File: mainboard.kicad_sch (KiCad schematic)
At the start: 15 parts, among them IC1 AZ1117CH-3.3TRG1, P1 OKLT6W12NC, U1 MCP2517FD-xSL, U5 MCP2517FD-xSL

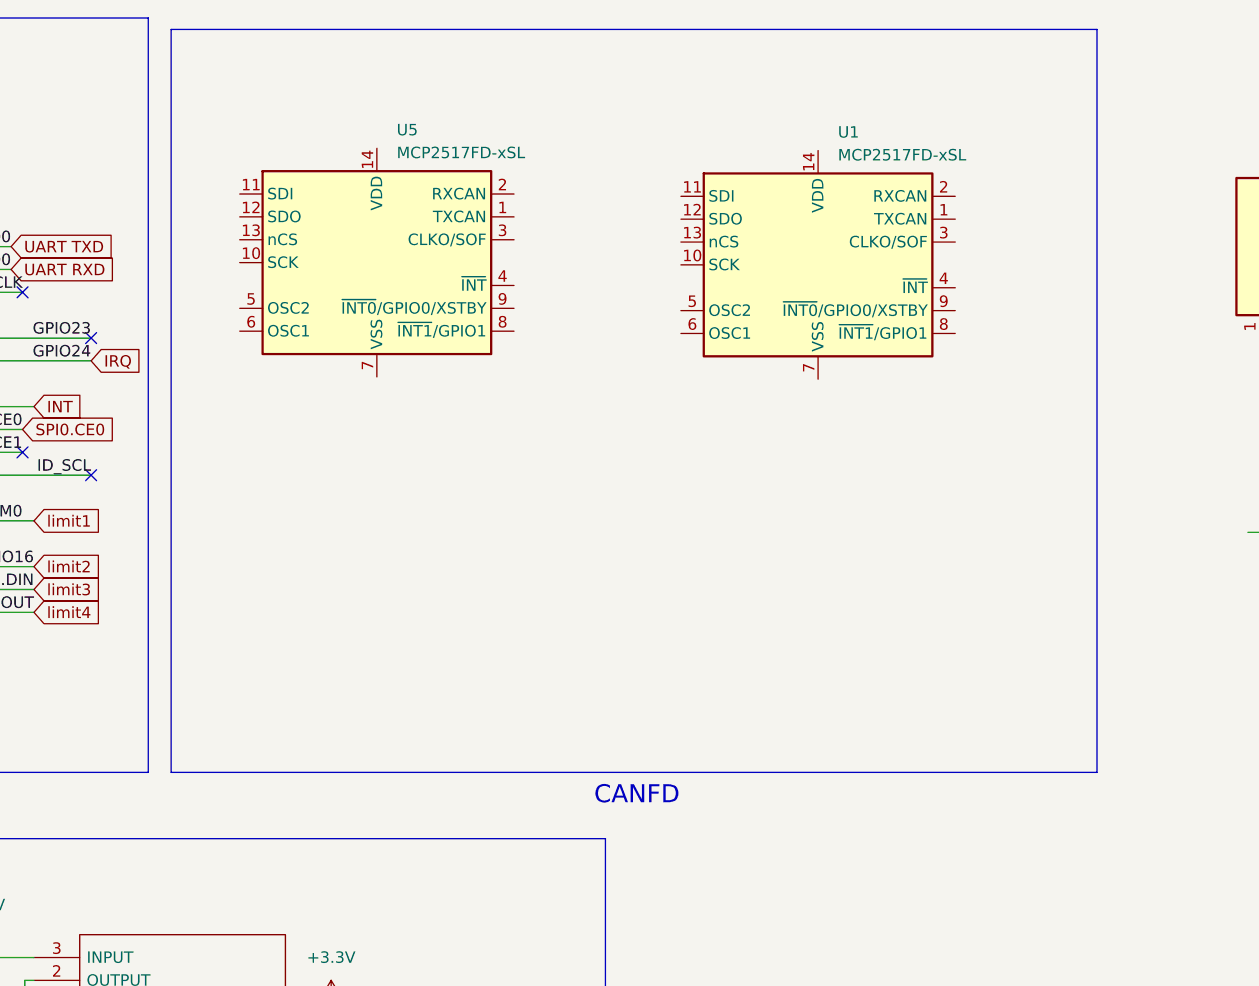
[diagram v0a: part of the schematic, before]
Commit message: 更新
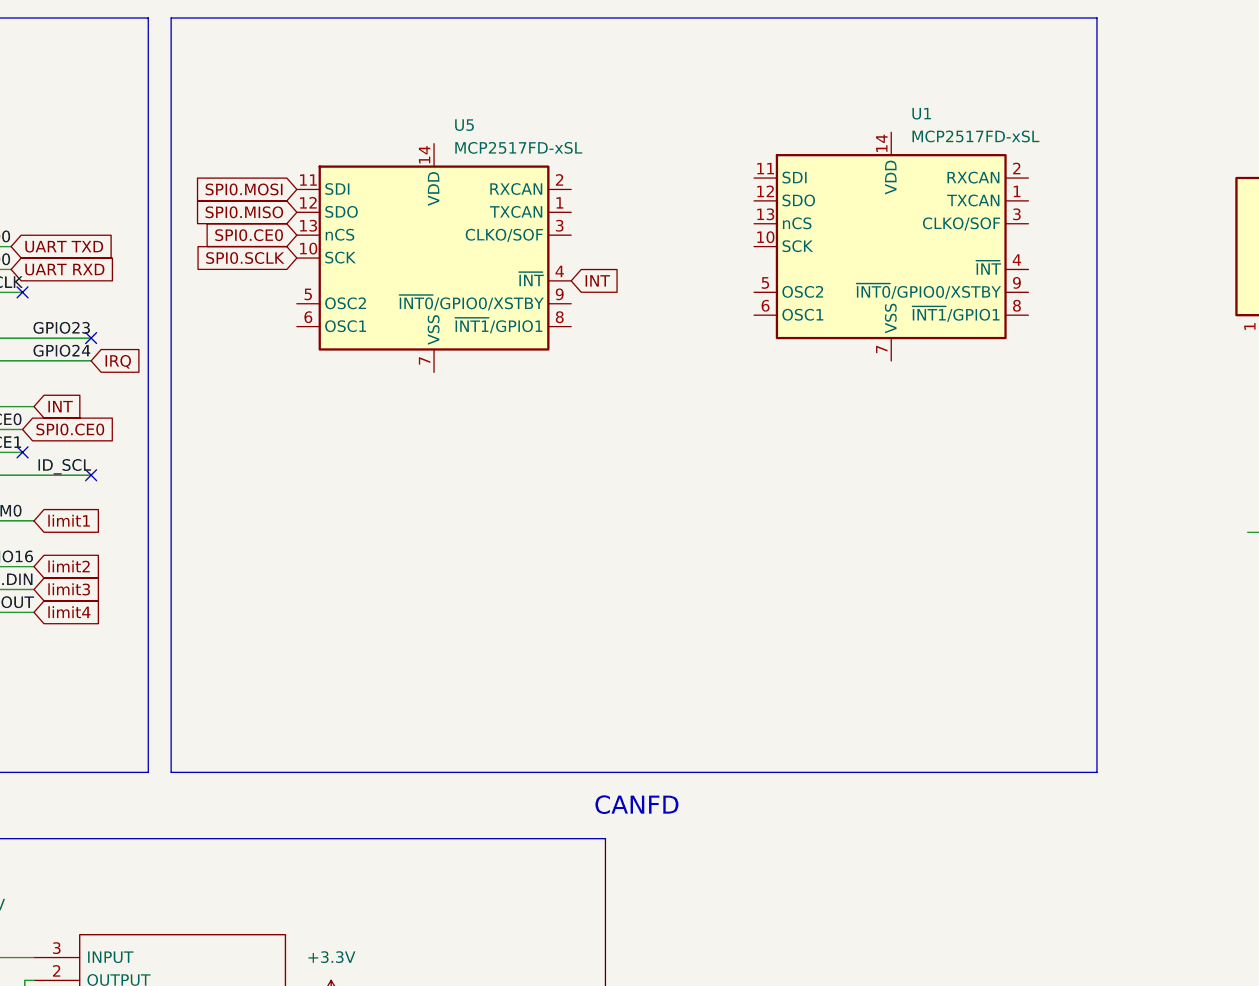
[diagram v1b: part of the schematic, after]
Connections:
- net INT: now also U5.4 (~{INT})
- net SPI0.CE0: now also U5.13 (nCS)
- net SPI0.MISO: now also U5.12 (SDO)
- net SPI0.MOSI: now also U5.11 (SDI)
- net SPI0.SCLK: now also U5.10 (SCK)
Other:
- moved on the sheet: U1, U5
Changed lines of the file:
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@@
     (fill (type none))
   )
-  (rectangle (start 100.33 19.05) (end 203.2 101.6)
+  (rectangle (start 100.33 17.78) (end 203.2 101.6)
     (stroke (width 0) (type default))
     (fill (type none))
@@
     (effects (font (size 2 2)) (justify left bottom))
   )
-  (text "CANFD" (at 147.32 105.41 0)
+  (text "CANFD" (at 147.32 106.68 0)
     (effects (font (size 2 2)) (justify left bottom))
   )
@@
     )
   )
+  (global_label "SPI0.SCLK" (shape input) (at 114.3 44.45 180) (fields_autoplaced)
+    (effects (font (size 1.27 1.27)) (justify right))
+    (property "Intersheetrefs" "${INTERSHEET_REFS}" (at 101.6386 44.45 0)
+      (effects (font (size 1.27 1.27)) (justify right) hide)
+    )
+  )
+  (global_label "INT" (shape input) (at 144.78 46.99 0) (fields_autoplaced)
+    (effects (font (size 1.27 1.27)) (justify left))
+    (property "Intersheetrefs" "${INTERSHEET_REFS}" (at 150.6681 46.99 0)
+      (effects (font (size 1.27 1.27)) (justify left) hide)
+    )
+  )
   (global_label "LED_R" (shape input) (at 22.86 50.8 180) (fields_autoplaced)
     (effects (font (size 1.27 1.27)) (justify right))
@@
     )
   )
+  (global_label "SPI0.CE0" (shape input) (at 114.3 41.91 180) (fields_autoplaced)
+    (effects (font (size 1.27 1.27)) (justify right))
+    (property "Intersheetrefs" "${INTERSHEET_REFS}" (at 102.7877 41.91 0)
+      (effects (font (size 1.27 1.27)) (justify right) hide)
+    )
+  )
+  (global_label "SPI0.MISO" (shape input) (at 114.3 39.37 180) (fields_autoplaced)
+    (effects (font (size 1.27 1.27)) (justify right))
+    (property "Intersheetrefs" "${INTERSHEET_REFS}" (at 101.82 39.37 0)
+      (effects (font (size 1.27 1.27)) (justify right) hide)
+    )
+  )
   (global_label "SPI0.CE0" (shape input) (at 83.82 63.5 0) (fields_autoplaced)
     (effects (font (size 1.27 1.27)) (justify left))
@@
     (property "Intersheetrefs" "${INTERSHEET_REFS}" (at 90.9781 60.96 0)
       (effects (font (size 1.27 1.27)) (justify left) hide)
+    )
+  )
+  (global_label "SPI0.MOSI" (shape input) (at 114.3 36.83 180) (fields_autoplaced)
+    (effects (font (size 1.27 1.27)) (justify right))
+    (property "Intersheetrefs" "${INTERSHEET_REFS}" (at 101.82 36.83 0)
+      (effects (font (size 1.27 1.27)) (justify right) hide)
     )
   )
@@
     )
   )
-  (symbol (lib_id "Interface_CAN_LIN:MCP2517FD-xSL") (at 172.212 45.212 0) (unit 1)
-    (in_bom yes) (on_board yes) (dnp no) (fields_autoplaced)
-    (property "Reference" "U1" (at 174.4061 30.48 0)
-      (effects (font (size 1.27 1.27)) (justify left))
-    )
-    (property "Value" "MCP2517FD-xSL" (at 174.4061 33.02 0)
-      (effects (font (size 1.27 1.27)) (justify left))
-    )
-    (property "Footprint" "Package_SO:SOIC-14_3.9x8.7mm_P1.27mm" (at 172.212 70.612 0)
-      (effects (font (size 1.27 1.27)) hide)
-    )
-    (property "Datasheet" "https://ww1.microchip.com/downloads/en/DeviceDoc/20005688A.pdf" (at 172.212 38.862 0)
+  (symbol (lib_id "Interface_CAN_LIN:MCP2517FD-xSL") (at 180.34 43.18 0) (unit 1)
+    (in_bom yes) (on_board yes) (dnp no) (fields_autoplaced)
+    (property "Reference" "U1" (at 182.5341 28.448 0)
+      (effects (font (size 1.27 1.27)) (justify left))
+    )
+    (property "Value" "MCP2517FD-xSL" (at 182.5341 30.988 0)
+      (effects (font (size 1.27 1.27)) (justify left))
+    )
+    (property "Footprint" "Package_SO:SOIC-14_3.9x8.7mm_P1.27mm" (at 180.34 68.58 0)
+      (effects (font (size 1.27 1.27)) hide)
+    )
+    (property "Datasheet" "https://ww1.microchip.com/downloads/en/DeviceDoc/20005688A.pdf" (at 180.34 36.83 0)
       (effects (font (size 1.27 1.27)) hide)
     )
@@
     )
   )
-  (symbol (lib_id "Interface_CAN_LIN:MCP2517FD-xSL") (at 123.19 44.958 0) (unit 1)
-    (in_bom yes) (on_board yes) (dnp no) (fields_autoplaced)
-    (property "Reference" "U5" (at 125.3841 30.226 0)
-      (effects (font (size 1.27 1.27)) (justify left))
-    )
-    (property "Value" "MCP2517FD-xSL" (at 125.3841 32.766 0)
-      (effects (font (size 1.27 1.27)) (justify left))
-    )
-    (property "Footprint" "Package_SO:SOIC-14_3.9x8.7mm_P1.27mm" (at 123.19 70.358 0)
-      (effects (font (size 1.27 1.27)) hide)
-    )
-    (property "Datasheet" "https://ww1.microchip.com/downloads/en/DeviceDoc/20005688A.pdf" (at 123.19 38.608 0)
-      (effects (font (size 1.27 1.27)) hide)
-    )
+  (symbol (lib_id "Interface_CAN_LIN:MCP2517FD-xSL") (at 129.54 44.45 0) (unit 1)
+    (in_bom yes) (on_board yes) (dnp no) (fields_autoplaced)
+    (property "Reference" "U5" (at 131.7341 29.718 0)
+      (effects (font (size 1.27 1.27)) (justify left))
+    )
+    (property "Value" "MCP2517FD-xSL" (at 131.7341 32.258 0)
+      (effects (font (size 1.27 1.27)) (justify left))
+    )
+    (property "Footprint" "Package_SO:SOIC-14_3.9x8.7mm_P1.27mm" (at 129.54 69.85 0)
+      (effects (font (size 1.27 1.27)) hide)
+    )
+    (property "Datasheet" "https://ww1.microchip.com/downloads/en/DeviceDoc/20005688A.pdf" (at 129.54 38.1 0)
+      (effects (font (size 1.27 1.27)) hide)
+    )
